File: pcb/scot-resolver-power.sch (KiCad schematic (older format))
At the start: 30 parts, among them IC4 TSR1, U1 MCP1703A-5002_SOT223, U2 LT1762, U3 MCP1703A-5002_SOT223, U4 MCP1703A-5002_SOT223, U5 MCP1703A-3302_SOT223

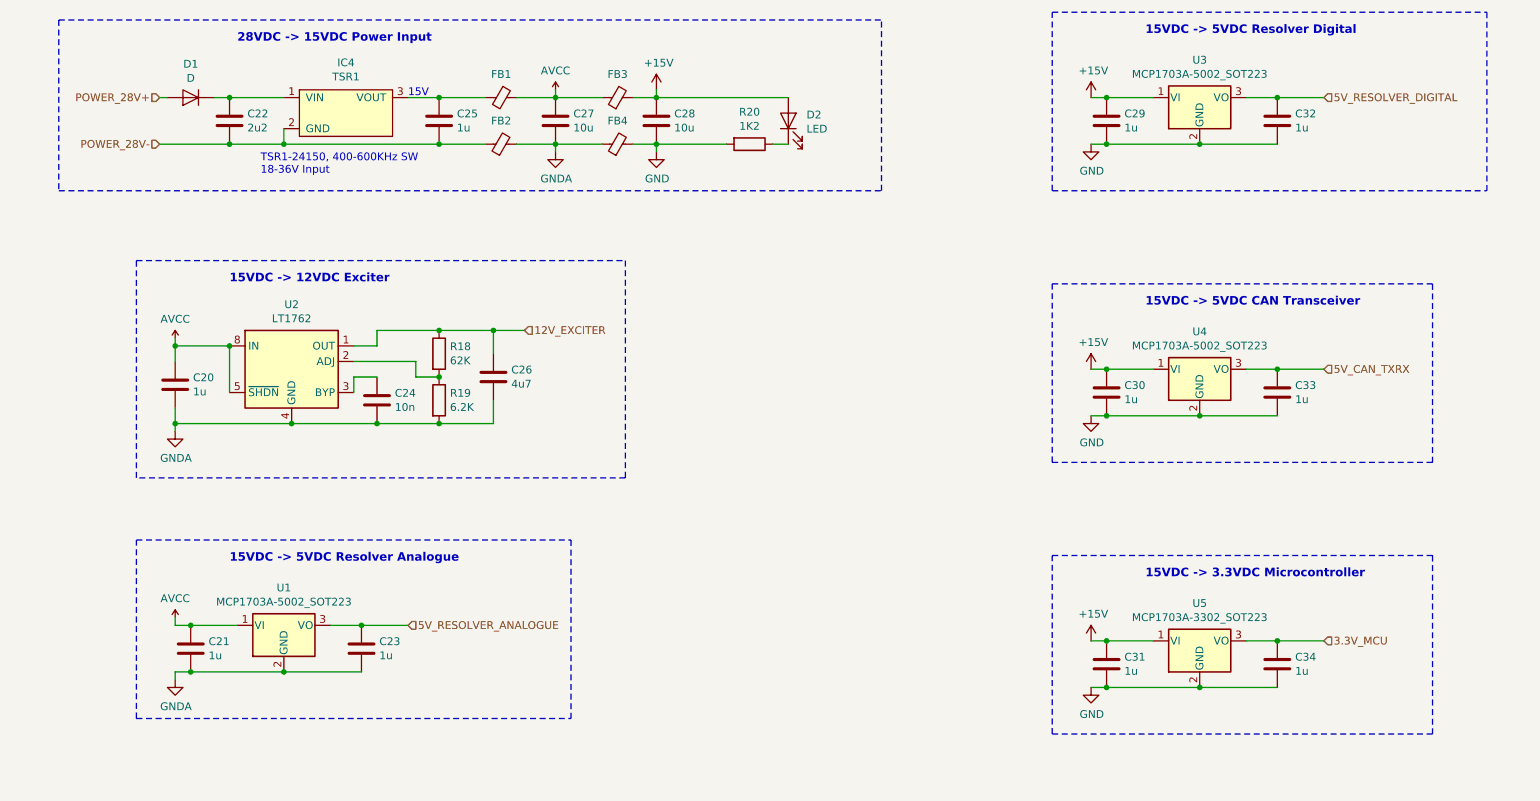
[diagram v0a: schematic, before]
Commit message: WIP PCB v2.
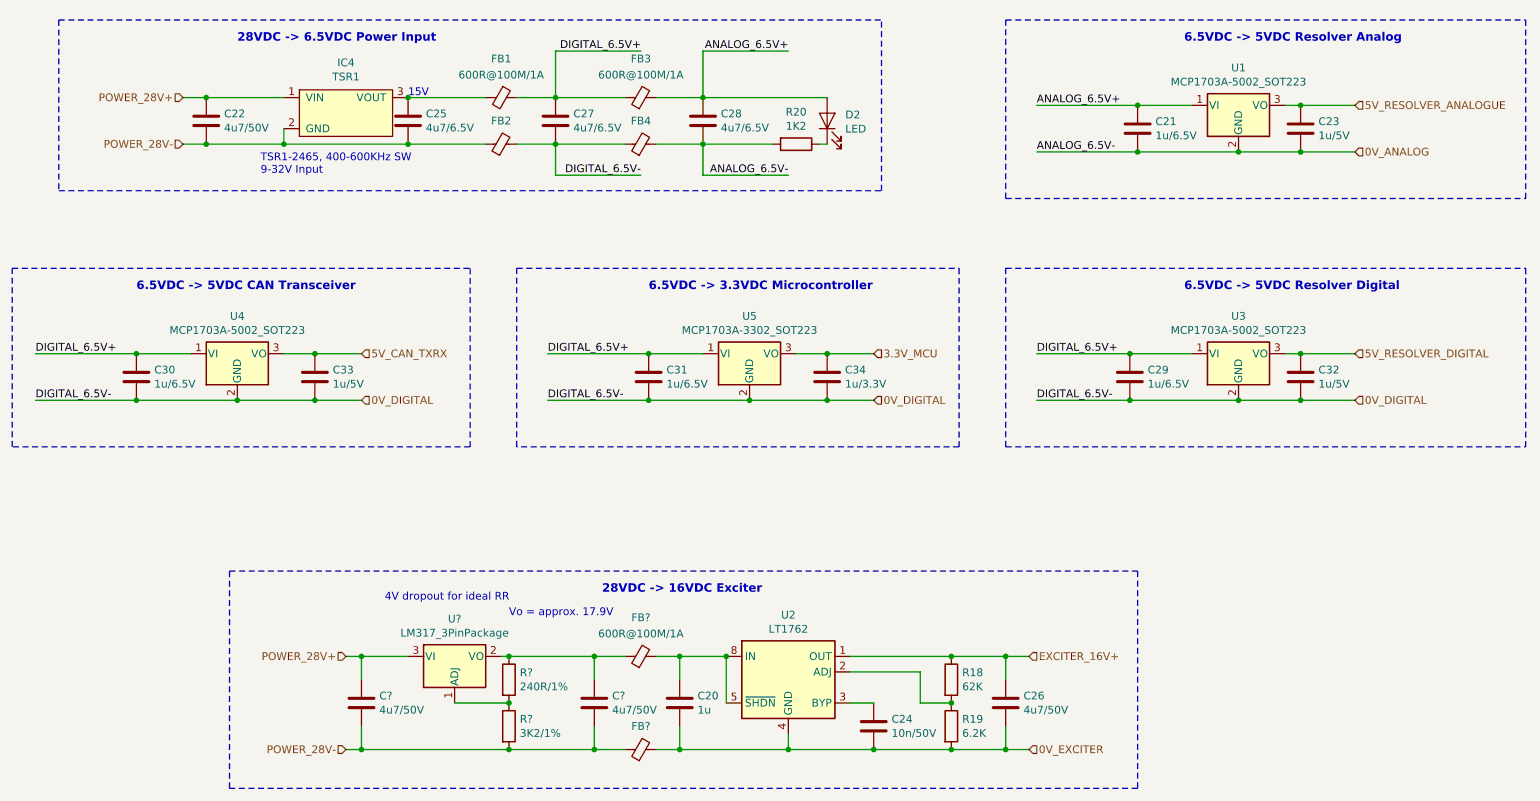
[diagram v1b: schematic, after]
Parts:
- removed D1: D, Diode_SMD:D_1206_3216Metric_Pad1.42x1.75mm_HandSolder, symbol Device:D
- added C?: 4u7/50V, Capacitor_SMD:C_1206_3216Metric_Pad1.42x1.75mm_HandSolder, symbol Device:C
- added C?: 4u7/50V, Capacitor_SMD:C_0603_1608Metric_Pad1.05x0.95mm_HandSolder, symbol Device:C
- added FB? (x2): 600R@100M/1A, Inductor_SMD:L_0805_2012Metric_Pad1.15x1.40mm_HandSolder, symbol Device:Ferrite_Bead_Small
- added R?: 240R/1%, Resistor_SMD:R_0805_2012Metric_Pad1.15x1.40mm_HandSolder, symbol Device:R
- added R?: 3K2/1%, Resistor_SMD:R_0805_2012Metric_Pad1.15x1.40mm_HandSolder, symbol Device:R
- added U?: LM317_3PinPackage, symbol Regulator_Linear:LM317_3PinPackage
- C21, C29, C30, C31: value 1u -> 1u/6.5V
- C22: value 2u2 -> 4u7/50V; footprint Capacitor_SMD:C_0603_1608Metric_Pad1.05x0.95mm_HandSolder -> Capacitor_SMD:C_1206_3216Metric_Pad1.42x1.75mm_HandSolder
- C23, C32, C33: value 1u -> 1u/5V
- C24: value 10n -> 10n/50V; footprint Capacitor_SMD:C_0402_1005Metric -> Capacitor_SMD:C_0603_1608Metric_Pad1.05x0.95mm_HandSolder
- C25: value 1u -> 4u7/6.5V
- C26: value 4u7 -> 4u7/50V
- C27, C28: value 10u -> 4u7/6.5V
- C34: value 1u -> 1u/3.3V
- FB1, FB2, FB3, FB4: value Ferrite_Bead_Small -> 600R@100M/1A
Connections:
- net POWER_28V+: now also C22.1, IC4.1 (VIN), C?.1, U?.3 (VI)
- net POWER_28V-: now also C?.2, C?.2, FB?.1, R?.2
- net +15V renamed DIGITAL_6.5V+
- net DIGITAL_6.5V+: now also C27.1, FB1.1, FB3.1; no longer C28.1, D2.2 (A), FB3.2
- net 12V_EXCITER renamed EXCITER_16V+
- removed net AVCC: C20.1, C21.1, C27.1, FB1.1, FB3.1, U1.1 (VI), U2.5 (~SHDN), U2.8 (IN)
- net GND renamed 0V_DIGITAL
- net 0V_DIGITAL: now also C27.2, FB2.2, FB4.1; no longer C28.2, FB4.2, R20.2
- removed net GNDA: C20.2, C21.2, C23.2, C24.2, C26.2, C27.2, FB2.2, FB4.1, R19.2, U1.2 (GND), U2.4 (GND)
- new net: C20.1, FB?.2, U2.5 (~SHDN), U2.8 (IN)
- new net: R?.1, R?.2, U?.1 (ADJ)
- new net: C?.1, FB?.1, R?.1, U?.2 (VO)
- new net 0V_ANALOG: C21.2, C23.2, C28.2, FB4.2, R20.2, U1.2 (GND)
- new net 0V_EXCITER: C20.2, C24.2, C26.2, FB?.2, R19.2, U2.4 (GND)
- new net ANALOG_6.5V+: C21.1, C28.1, D2.2 (A), FB3.2, U1.1 (VI)
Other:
- note added: "28VDC -> 16VDC Exciter"
- note added: "28VDC -> 6.5VDC Power Input"
- note added: "4V dropout for ideal RR"
- note added: "6.5VDC -> 3.3VDC Microcontroller"
- note added: "6.5VDC -> 5VDC CAN Transceiver"
- note added: "6.5VDC -> 5VDC Resolver Analog"
- note added: "6.5VDC -> 5VDC Resolver Digital"
- note added: "TSR1-2465, 400-600KHz SW\n9-32V Input"
- note added: "Vo = approx. 17.9V"
- note removed: "15VDC -> 12VDC Exciter"
- note removed: "15VDC -> 3.3VDC Microcontroller"
- note removed: "15VDC -> 5VDC CAN Transceiver"
- note removed: "15VDC -> 5VDC Resolver Analogue"
- note removed: "15VDC -> 5VDC Resolver Digital"
- note removed: "28VDC -> 15VDC Power Input"
- note removed: "TSR1-24150, 400-600KHz SW\n18-36V Input"
- moved on the sheet: C20, C21, C22, C23, C24, C25, C26, C28, C29, C30, C31, C32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
